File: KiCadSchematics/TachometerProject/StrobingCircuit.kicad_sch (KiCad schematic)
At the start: 9 parts

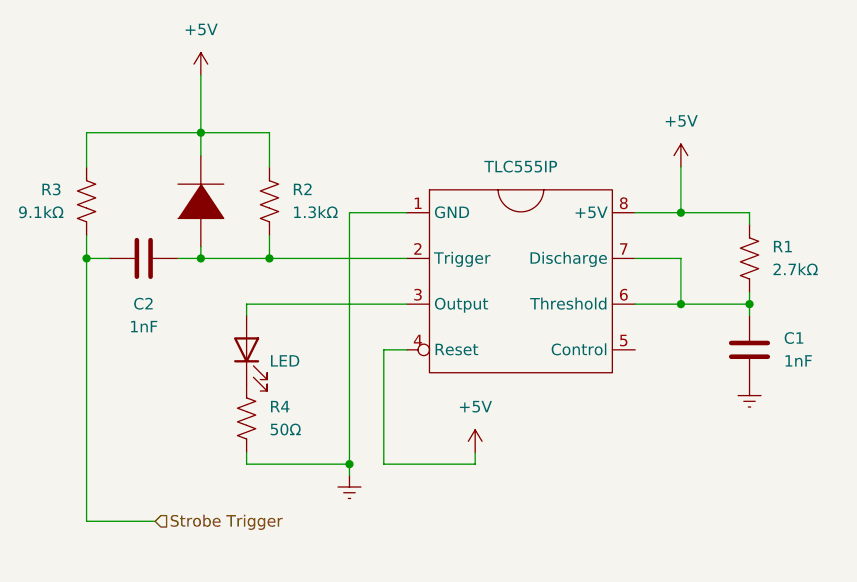
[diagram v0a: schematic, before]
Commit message: Updated circuit diagrams
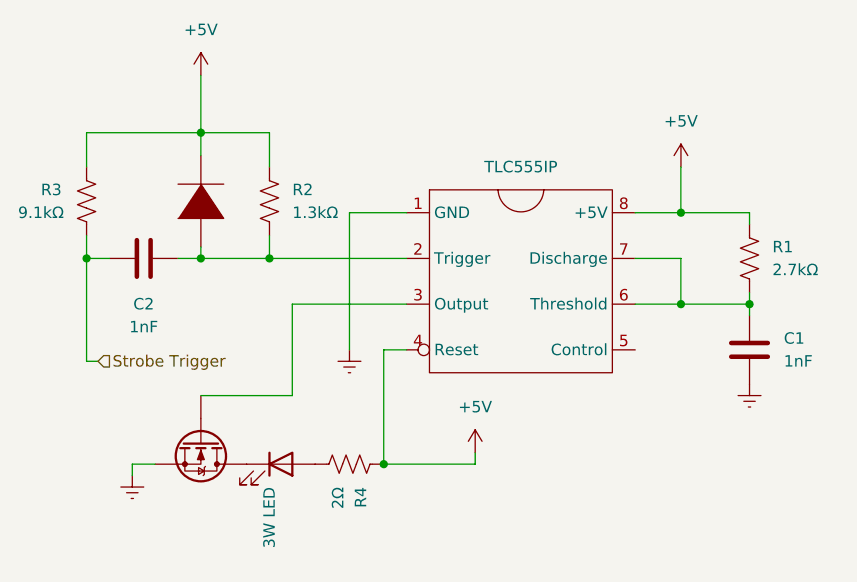
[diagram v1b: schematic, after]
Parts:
- added Q?: Q_NMOS_GDS, symbol Device:Q_NMOS_GDS
- D?: value LED -> 3W LED
- R4: value 50Ω -> 2Ω
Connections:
- net +5V: now also R4.1
- net Earth: now also Q?.3 (S); no longer R4.2
- net at D?.1 (K): now also Q?.2 (D); no longer R4.1
- net at D?.2 (A): now also R4.2; no longer U?.3 (Output)
- new net: Q?.1 (G), U?.3 (Output)
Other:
- moved on the sheet: R4
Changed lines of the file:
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@@
   (junction (at 161.29 82.55) (diameter 0) (color 0 0 0 0)
   )
+  (junction (at 128.27 110.49) (diameter 0) (color 0 0 0 0)
+  )
   (junction (at 107.95 87.63) (diameter 0) (color 0 0 0 0)
   )
@@
   (junction (at 168.91 92.71) (diameter 0) (color 0 0 0 0)
   )
-  (junction (at 124.46 110.49) (diameter 0) (color 0 0 0 0)
-  )
   (junction (at 107.95 73.66) (diameter 0) (color 0 0 0 0)
   )
@@
     (stroke (width 0) (type default) (color 0 0 0 0))
   )
-  (wire (pts (xy 95.25 87.63) (xy 95.25 116.84))
+  (wire (pts (xy 95.25 87.63) (xy 95.25 99.06))
     (stroke (width 0) (type default) (color 0 0 0 0))
   )
@@
     (stroke (width 0) (type default) (color 0 0 0 0))
   )
+  (wire (pts (xy 102.87 110.49) (xy 100.33 110.49))
+    (stroke (width 0) (type default) (color 0 0 0 0))
+  )
   (wire (pts (xy 95.25 73.66) (xy 107.95 73.66))
     (stroke (width 0) (type default) (color 0 0 0 0))
   )
-  (wire (pts (xy 113.03 109.22) (xy 113.03 110.49))
+  (wire (pts (xy 118.11 92.71) (xy 118.11 102.87))
     (stroke (width 0) (type default) (color 0 0 0 0))
   )
@@
     (stroke (width 0) (type default) (color 0 0 0 0))
   )
+  (wire (pts (xy 100.33 110.49) (xy 100.33 111.76))
+    (stroke (width 0) (type default) (color 0 0 0 0))
+  )
   (wire (pts (xy 138.43 110.49) (xy 128.27 110.49))
     (stroke (width 0) (type default) (color 0 0 0 0))
@@
     (stroke (width 0) (type default) (color 0 0 0 0))
   )
-  (wire (pts (xy 113.03 110.49) (xy 124.46 110.49))
+  (wire (pts (xy 130.81 92.71) (xy 118.11 92.71))
     (stroke (width 0) (type default) (color 0 0 0 0))
   )
@@
     (stroke (width 0) (type default) (color 0 0 0 0))
   )
-  (wire (pts (xy 124.46 82.55) (xy 124.46 110.49))
+  (wire (pts (xy 124.46 82.55) (xy 124.46 97.79))
     (stroke (width 0) (type default) (color 0 0 0 0))
   )
@@
     (stroke (width 0) (type default) (color 0 0 0 0))
   )
-  (wire (pts (xy 130.81 92.71) (xy 113.03 92.71))
-    (stroke (width 0) (type default) (color 0 0 0 0))
-  )
-  (wire (pts (xy 95.25 116.84) (xy 102.87 116.84))
-    (stroke (width 0) (type default) (color 0 0 0 0))
-  )
-  (wire (pts (xy 124.46 111.76) (xy 124.46 110.49))
+  (wire (pts (xy 95.25 99.06) (xy 96.52 99.06))
+    (stroke (width 0) (type default) (color 0 0 0 0))
+  )
+  (wire (pts (xy 118.11 102.87) (xy 107.95 102.87))
     (stroke (width 0) (type default) (color 0 0 0 0))
   )
@@
     (stroke (width 0) (type default) (color 0 0 0 0))
   )
-  (wire (pts (xy 113.03 92.71) (xy 113.03 93.98))
-    (stroke (width 0) (type default) (color 0 0 0 0))
-  )
-  (hierarchical_label "Strobe Trigger" (shape input) (at 102.87 116.84 0)
+  (hierarchical_label "Strobe Trigger" (shape input) (at 96.52 99.06 0)
     (effects (font (size 1.27 1.27)) (justify left))
   )
@@
     (pin "2")
   )
-  (symbol (lib_id "Device:LED") (at 113.03 97.79 90) (unit 1)
+  (symbol (lib_id "Device:LED") (at 116.84 110.49 0) (unit 1)
     (in_bom yes) (on_board yes)
-    (property "Reference" "D?" (id 0) (at 116.84 98.1074 90)
+    (property "Reference" "D?" (id 0) (at 116.5226 114.3 90)
       (effects (font (size 1.27 1.27)) (justify right) hide)
     )
-    (property "Value" "LED" (id 1) (at 115.57 99.06 90)
+    (property "Value" "3W LED" (id 1) (at 115.57 113.03 90)
       (effects (font (size 1.27 1.27)) (justify right))
     )
-    (property "Footprint" "" (id 2) (at 113.03 97.79 0)
-      (effects (font (size 1.27 1.27)) hide)
-    )
-    (property "Datasheet" "~" (id 3) (at 113.03 97.79 0)
+    (property "Footprint" "" (id 2) (at 116.84 110.49 0)
+      (effects (font (size 1.27 1.27)) hide)
+    )
+    (property "Datasheet" "~" (id 3) (at 116.84 110.49 0)
       (effects (font (size 1.27 1.27)) hide)
     )
@@
     (pin "1")
   )
-  (symbol (lib_id "Device:R_US") (at 113.03 105.41 0) (unit 1)
-    (in_bom yes) (on_board yes) (fields_autoplaced)
-    (property "Reference" "R4" (id 0) (at 115.57 104.1399 0)
-      (effects (font (size 1.27 1.27)) (justify left))
-    )
-    (property "Value" "50Ω" (id 1) (at 115.57 106.6799 0)
-      (effects (font (size 1.27 1.27)) (justify left))
-    )
-    (property "Footprint" "" (id 2) (at 114.046 105.664 90)
-      (effects (font (size 1.27 1.27)) hide)
-    )
-    (property "Datasheet" "~" (id 3) (at 113.03 105.41 0)
-      (effects (font (size 1.27 1.27)) hide)
-    )
-    (pin "1")
-    (pin "2")
-  )
-  (symbol (lib_id "power:Earth") (at 124.46 111.76 0) (unit 1)
-    (in_bom yes) (on_board yes) (fields_autoplaced)
-    (property "Reference" "#PWR?" (id 0) (at 124.46 118.11 0)
-      (effects (font (size 1.27 1.27)) hide)
-    )
-    (property "Value" "Earth" (id 1) (at 124.46 115.57 0)
-      (effects (font (size 1.27 1.27)) hide)
-    )
-    (property "Footprint" "" (id 2) (at 124.46 111.76 0)
-      (effects (font (size 1.27 1.27)) hide)
-    )
-    (property "Datasheet" "~" (id 3) (at 124.46 111.76 0)
-      (effects (font (size 1.27 1.27)) hide)
-    )
+  (symbol (lib_id "Device:Q_NMOS_GDS") (at 107.95 107.95 270) (unit 1)
+    (in_bom yes) (on_board yes) (fields_autoplaced)
+    (property "Reference" "Q?" (id 0) (at 107.95 115.57 90)
+      (effects (font (size 1.27 1.27)) hide)
+    )
+    (property "Value" "Q_NMOS_GDS" (id 1) (at 107.95 115.57 90)
+      (effects (font (size 1.27 1.27)) hide)
+    )
+    (property "Footprint" "" (id 2) (at 110.49 113.03 0)
+      (effects (font (size 1.27 1.27)) hide)
+    )
+    (property "Datasheet" "~" (id 3) (at 107.95 107.95 0)
+      (effects (font (size 1.27 1.27)) hide)
+    )
+    (pin "1")
+    (pin "2")
+    (pin "3")
+  )
+  (symbol (lib_id "Device:R_US") (at 124.46 110.49 270) (unit 1)
+    (in_bom yes) (on_board yes) (fields_autoplaced)
+    (property "Reference" "R4" (id 0) (at 125.7301 113.03 0)
+      (effects (font (size 1.27 1.27)) (justify left))
+    )
+    (property "Value" "2Ω" (id 1) (at 123.1901 113.03 0)
+      (effects (font (size 1.27 1.27)) (justify left))
+    )
+    (property "Footprint" "" (id 2) (at 124.206 111.506 90)
+      (effects (font (size 1.27 1.27)) hide)
+    )
+    (property "Datasheet" "~" (id 3) (at 124.46 110.49 0)
+      (effects (font (size 1.27 1.27)) hide)
+    )
+    (pin "1")
+    (pin "2")
+  )
+  (symbol (lib_id "power:Earth") (at 124.46 97.79 0) (unit 1)
+    (in_bom yes) (on_board yes) (fields_autoplaced)
+    (property "Reference" "#PWR?" (id 0) (at 124.46 104.14 0)
+      (effects (font (size 1.27 1.27)) hide)
+    )
+    (property "Value" "Earth" (id 1) (at 124.46 101.6 0)
+      (effects (font (size 1.27 1.27)) hide)
+    )
+    (property "Footprint" "" (id 2) (at 124.46 97.79 0)
+      (effects (font (size 1.27 1.27)) hide)
+    )
+    (property "Datasheet" "~" (id 3) (at 124.46 97.79 0)
+      (effects (font (size 1.27 1.27)) hide)
+    )
+    (pin "1")
+  )
+  (symbol (lib_id "power:Earth") (at 100.33 111.76 0) (unit 1)
+    (in_bom yes) (on_board yes) (fields_autoplaced)
+    (property "Reference" "#PWR?" (id 0) (at 100.33 118.11 0)
+      (effects (font (size 1.27 1.27)) hide)
+    )
+    (property "Value" "Earth" (id 1) (at 100.33 115.57 0)
+      (effects (font (size 1.27 1.27)) hide)
+    )
+    (property "Footprint" "" (id 2) (at 100.33 111.76 0)
+      (effects (font (size 1.27 1.27)) hide)
+    )
+    (property "Datasheet" "~" (id 3) (at 100.33 111.76 0)
+      (effects (font (size 1.27 1.27)) hide)
+    )
